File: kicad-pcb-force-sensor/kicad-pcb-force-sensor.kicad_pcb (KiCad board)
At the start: 2 copper layers, 68.6 x 53.3 mm, 25 parts, among them J1 Power, J2 Digital/PWM, J3 Analog, J4 Digital/PWM, M1 Motor_Servo, U3 KY-040

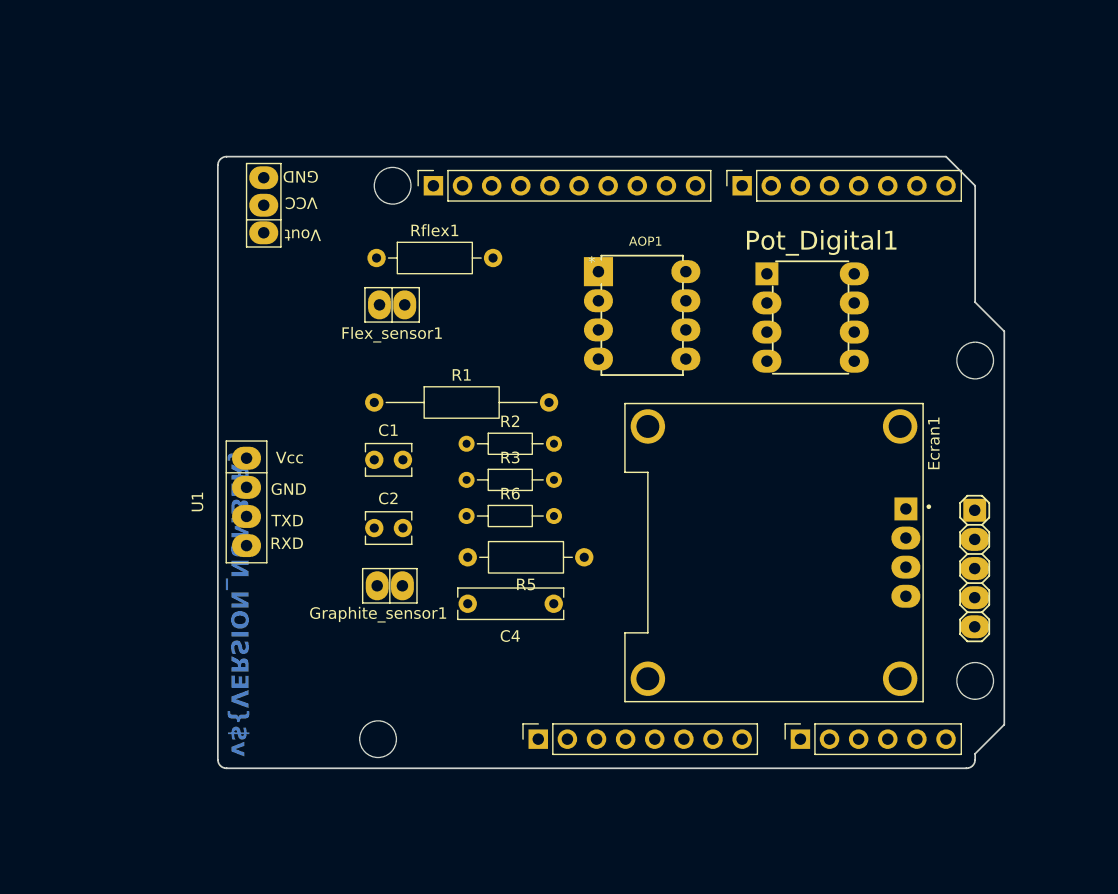
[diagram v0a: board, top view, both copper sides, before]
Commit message: Avec pistes
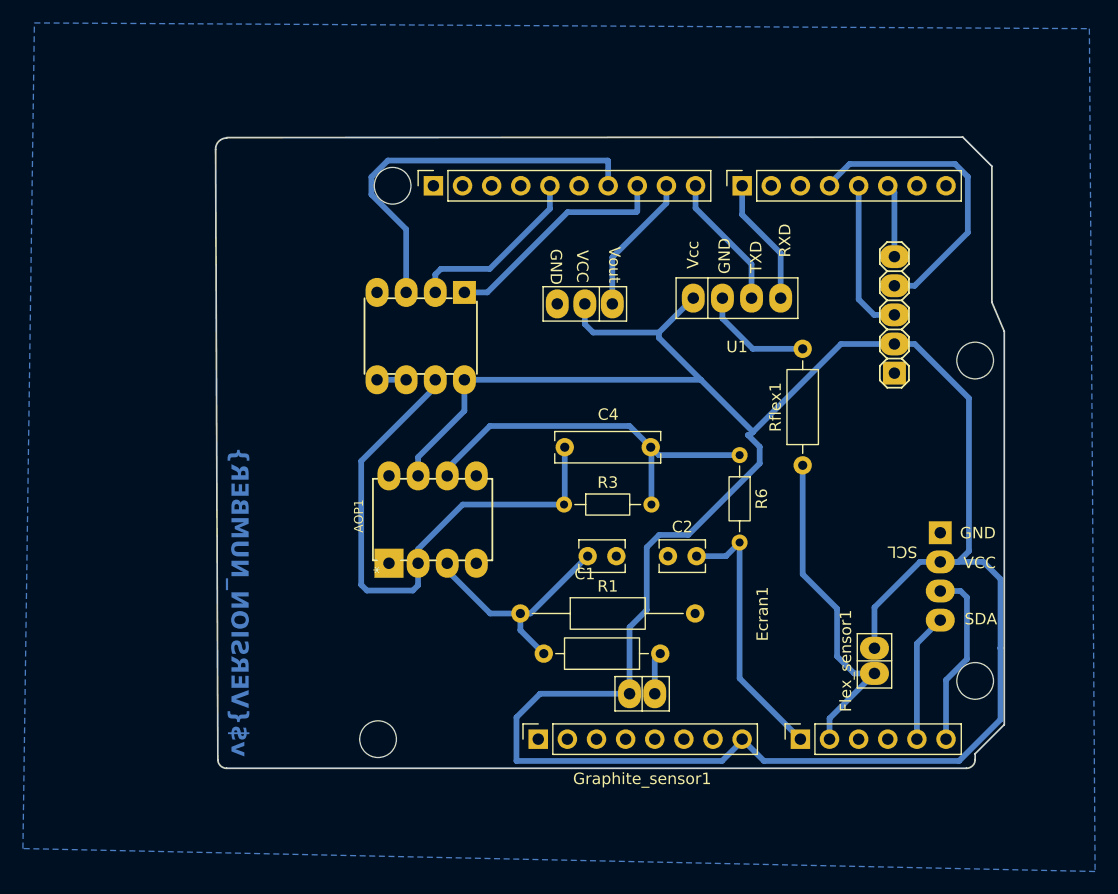
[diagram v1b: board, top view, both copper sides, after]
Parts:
- removed R2: 1k, Resistor_THT:R_Axial_DIN0204_L3.6mm_D1.6mm_P7.62mm_Horizontal
- AOP1: value LTC1050HS8_PBF -> LTC1050
- Rflex1: value 23k -> 47k
- moved Flex_sensor1 52.3 mm to (157.3, 90.6), turned to -90 degrees
- moved U1 46.3 mm to (145.3, 59.0), turned to 0 degrees
- moved Pot_Digital1 41.7 mm to (113.9, 66.1), turned to -90 degrees
- moved Rflex1 41.3 mm to (151.0, 73.6), turned to 90 degrees
- moved M1 29.3 mm to (132.0, 59.5), turned to 180 degrees
- moved C2 25.7 mm to (139.2, 81.5)
- moved R6 24.4 mm to (145.5, 72.7), turned to -90 degrees
- moved Graphite_sensor1 23.9 mm to (137.0, 93.5)
- moved C1 22.7 mm to (134.8, 81.5), turned to 180 degrees
- moved R1 22.4 mm to (126.4, 86.5)
- moved C4 21.0 mm to (137.8, 72.0), turned to 180 degrees
- moved AOP1 20.9 mm to (122.5, 74.5), turned to 90 degrees
- moved U3 20.8 mm to (159.0, 61.7), turned to -90 degrees
- moved R5 18.8 mm to (138.6, 90.0), turned to 180 degrees
- moved R3 8.77 mm to (130.2, 77.0)
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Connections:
- J2 pad 8: D10 PWM/MOSI -> D10 PWM/SS
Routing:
- net VCC: track 0.00 -> 214.4 mm
- net R2: track 0.00 -> 48.4 mm
- net D11 PWM/MOSI: track 0.00 -> 34.7 mm
- net Net-(AOP1-OUT): track 0.00 -> 33.7 mm
- net Flex: track 0.00 -> 29.1 mm
- net DT: track 0.00 -> 26.6 mm
- net ADC: track 0.00 -> 23.6 mm
- net Net-(AOP1-+IN): track 0.00 -> 20.8 mm
- net D10 PWM/SS: track 0.00 -> 20.2 mm
- net D13 PWM/SCK: track 0.00 -> 15.9 mm
- net SCL: track 0.00 -> 15.7 mm
- net GND: track 0.00 -> 13.9 mm
- net SW: track 0.00 -> 13.6 mm
- net D9 PWM: track 0.00 -> 12.3 mm
- net TXD: track 0.00 -> 11.8 mm
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- added copper zone on B.Cu, net GND
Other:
- board size 68.6 x 53.3 mm -> 68.8 x 55 mm
- board text added: "SCL"
